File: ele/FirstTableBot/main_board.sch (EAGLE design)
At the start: 109 parts, among them IC1 MCP602ST, X4 POWER_IN

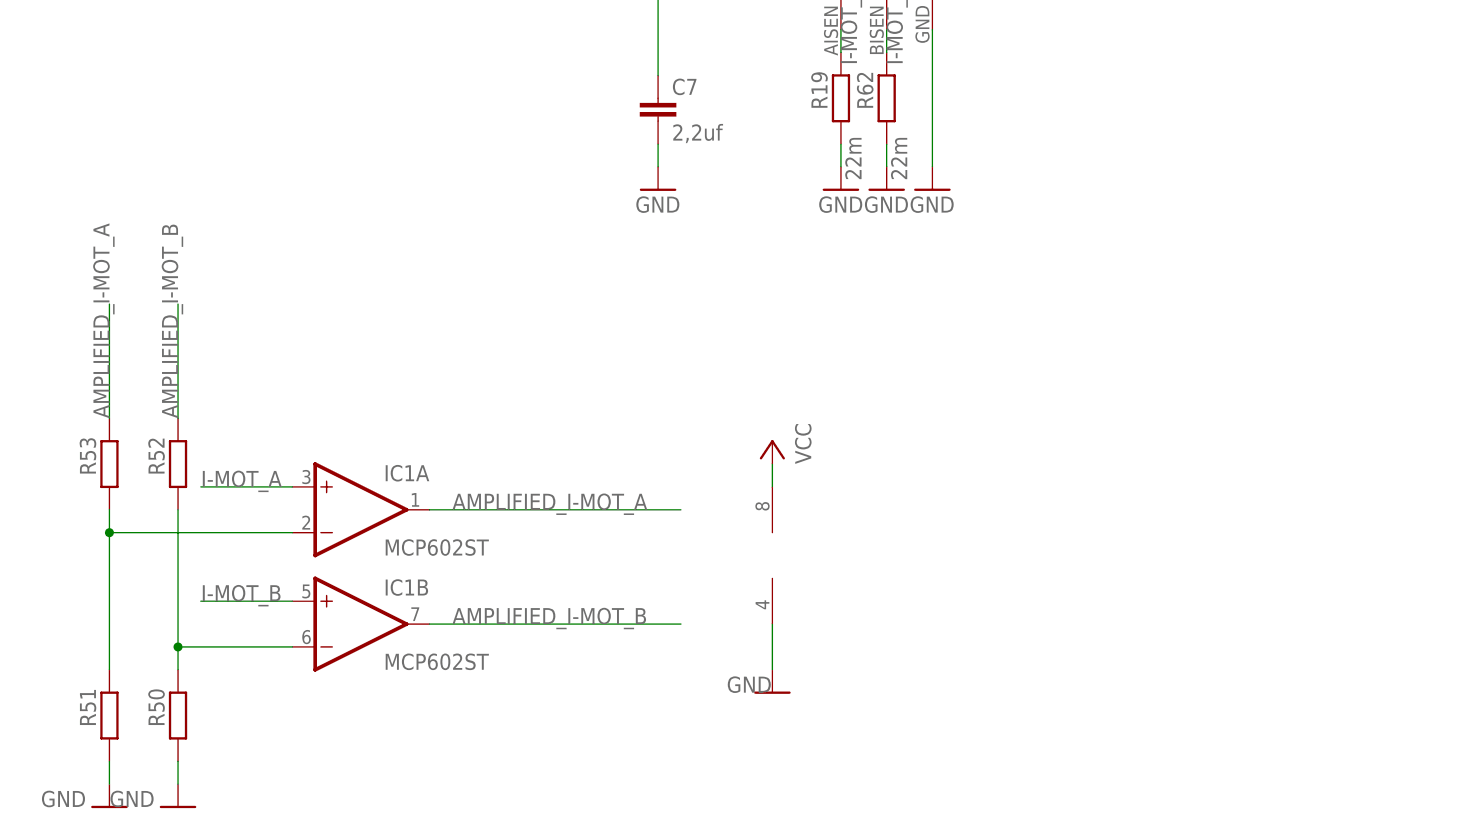
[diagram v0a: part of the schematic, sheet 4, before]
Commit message: dolni propust k zesilovacum
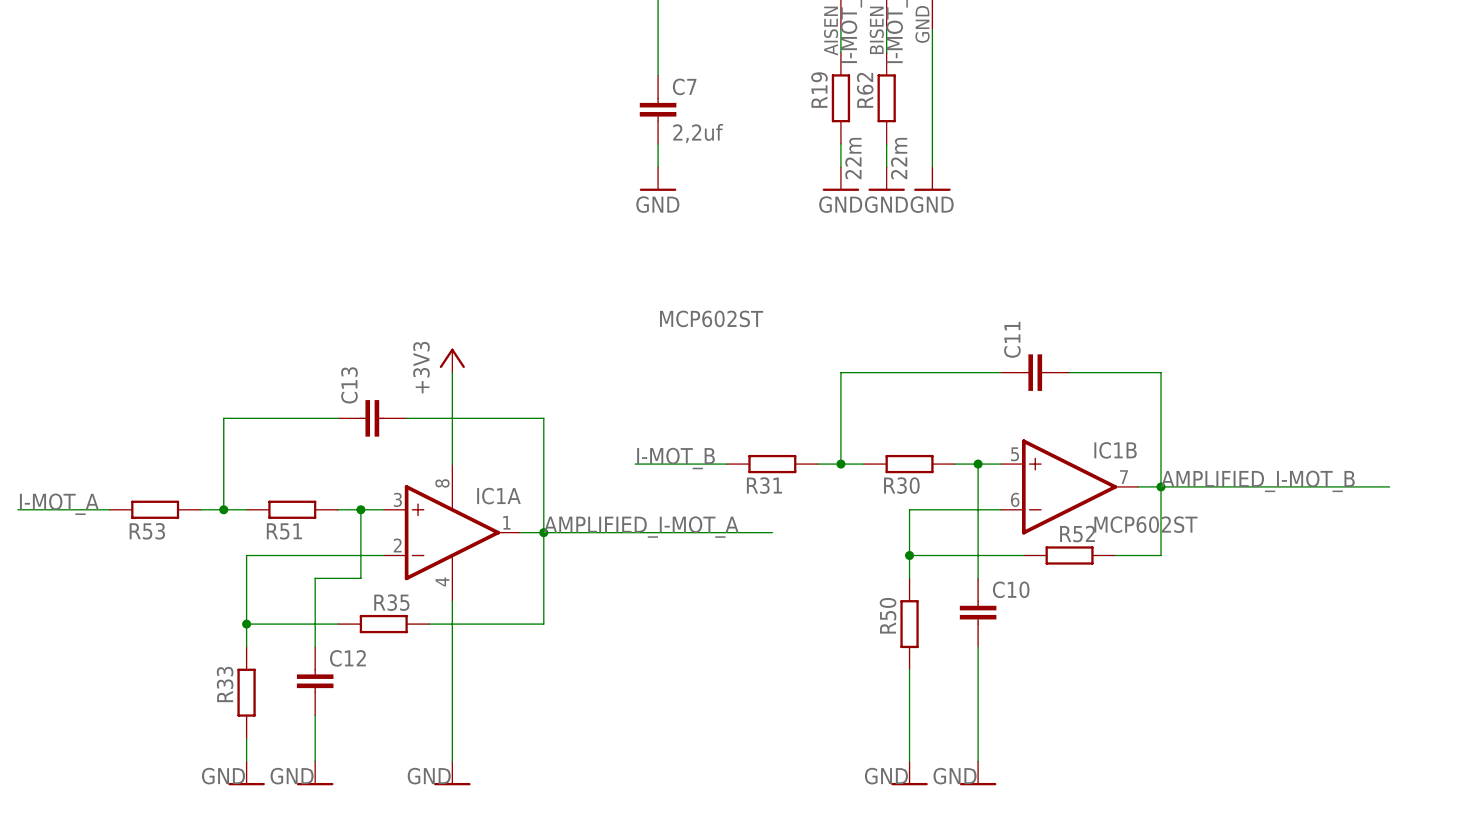
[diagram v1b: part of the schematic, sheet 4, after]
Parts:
- added C10, C11, C12, C13: (no value), resistor:C-EUC1206
- added R30, R31, R33, R35: (no value), resistor:R-EU_R0603
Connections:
- removed net N$29: IC1A.-IN, R51.2, R53.1
- new net N$18: C11.1, R30.2, R31.1
- new net N$19: C10.1, IC1B.+IN, R30.1
- new net N$20: IC1A.-IN, R33.2, R35.1
- new net N$32: C13.1, R51.2, R53.1
- new net N$33: C12.1, IC1A.+IN, R51.1
- net +3V3: now also IC1P.V+
- net AMPLIFIED_I-MOT_A: now also C13.2, R35.2; no longer R53.2
- net AMPLIFIED_I-MOT_B: now also C11.2
- net GND: now also C10.2, C12.2, R33.1; no longer R51.1
- net I-MOT_A: now also R53.2; no longer IC1A.+IN
- net I-MOT_B: now also R31.2; no longer IC1B.+IN
- net VCC: no longer IC1P.V+
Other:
- moved on the sheet: IC1A, IC1B, R50, R51, R52, R53

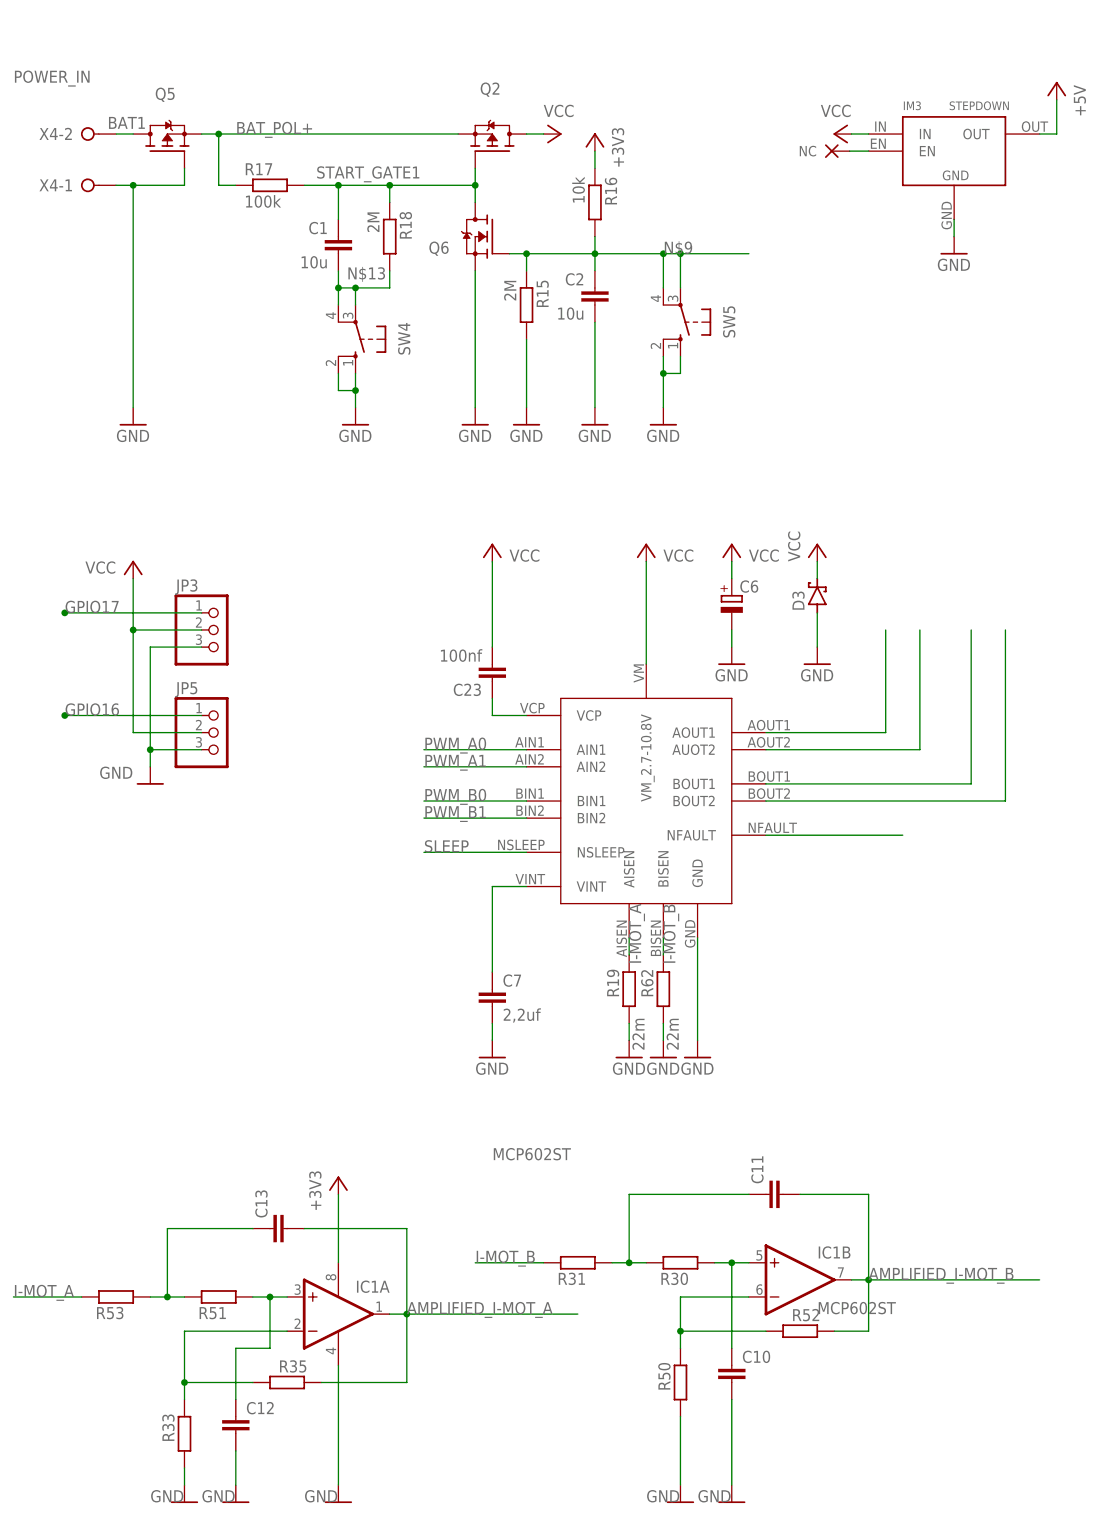
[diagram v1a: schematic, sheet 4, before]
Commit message: napajeni IR-led senzoru
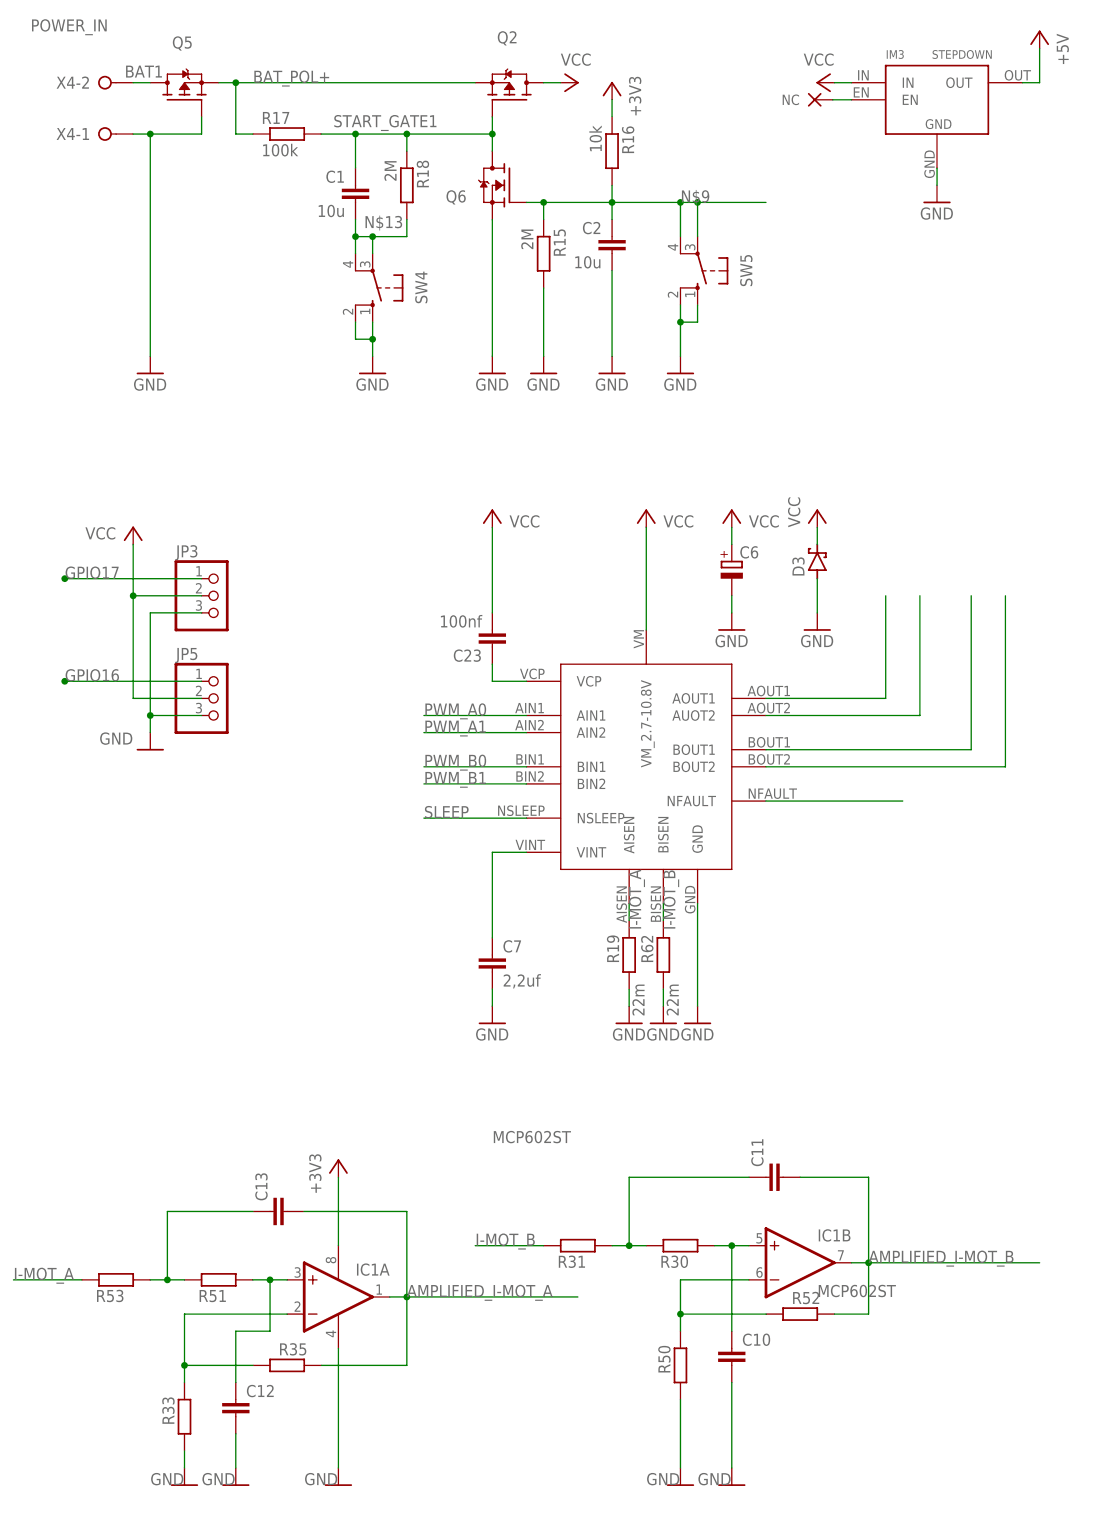
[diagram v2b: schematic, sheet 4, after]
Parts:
- removed R13, R3, R7: (no value), resistor:R-EU_R0603
- added Q8: (no value), transistors:P-MOSFET-MLP_HS
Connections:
- removed net N$7: R13.2, U$7.A
- new net N$29: U$6.C, U$7.A
- new net N$34: Q8.S, R1.1, R11.1, R5.1, R9.1
- net +5V: now also Q8.D
- net GND: no longer U$2.C, U$3.C, U$6.C
- net IR-LED-POWER: now also Q8.G; no longer R1.1, R11.1, R13.1, R3.1, R5.1, R7.1, R9.1
- net N$2: now also U$2.C; no longer R3.2
- net N$4: now also U$3.C; no longer R7.2
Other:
- moved on the sheet: C1, C10, C11, C12, C13, C2, C23, C6, C7, D3, IC1A, IC1B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

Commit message: piniste
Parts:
- added JP2, JP7, JP8: (no value), pinhead:PINHD-2X13
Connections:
- removed net GPIO21: Q3.S, R22.2
- removed net GPIO33: R20.S
- new net BAT-REF: IM6.IO33, R20.S
- new net I-LED: IM6.IO21, Q3.S, R22.2
- new net IO13: IM6.IO13, JP2.19, JP2.20
- new net IO14: IM6.IO14, JP2.17, JP2.18
- new net IO16: IM6.IO16, JP2.15, JP2.16
- new net IO17: IM6.IO17, JP2.13, JP2.14
- new net IO18: IM6.IO18, JP2.11, JP2.12
- new net IO19: IM6.IO19, JP2.10, JP2.9
- new net IO25: IM6.IO25, JP2.7, JP2.8
- new net IO26: IM6.IO26, JP2.5, JP2.6
- new net IO27: IM6.IO27, JP2.3, JP2.4
- new net IO32: IM6.IO32, JP2.1, JP2.2
- new net IO4: IM6.IO4, JP2.21, JP2.22
- new net RX: IM6.RXD0, JP2.25, JP2.26
- new net TX: IM6.TXD0, JP2.23, JP2.24
- net +3V3: now also JP7.10, JP7.12, JP7.14, JP7.16, JP7.18, JP7.2, JP7.20, JP7.22, JP7.24, JP7.26, JP7.4, JP7.6, JP7.8, JP8.10, JP8.12, JP8.14, JP8.16, JP8.18, JP8.2, JP8.20, JP8.22, JP8.24, JP8.26, JP8.4, JP8.6, JP8.8, R34.1, R37.1, R54.1, R55.1
- net +5V: no longer R34.1, R37.1, R54.1, R55.1
- net GND: now also JP7.1, JP7.11, JP7.13, JP7.15, JP7.17, JP7.19, JP7.21, JP7.23, JP7.25, JP7.3, JP7.5, JP7.7, JP7.9, JP8.1, JP8.11, JP8.13, JP8.15, JP8.17, JP8.19, JP8.21, JP8.23, JP8.25, JP8.3, JP8.5, JP8.7, JP8.9
- net PWM_A1: now also IM6.IO15; no longer IM6.IO16
- net PWM_B0: now also IM6.IO0; no longer IM6.IO17
- net SLEEP: now also IM6.IO2
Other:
- note added: "THIS SIGNAL MUST BE HERE!"
